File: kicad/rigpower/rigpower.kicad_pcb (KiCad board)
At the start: 2 copper layers, 66 x 54.6 mm, 16 parts, among them J1 Conn_01x02, J2 Conn_01x02, J3 Conn_01x02, J4 Conn_01x02, J5 Conn_01x02

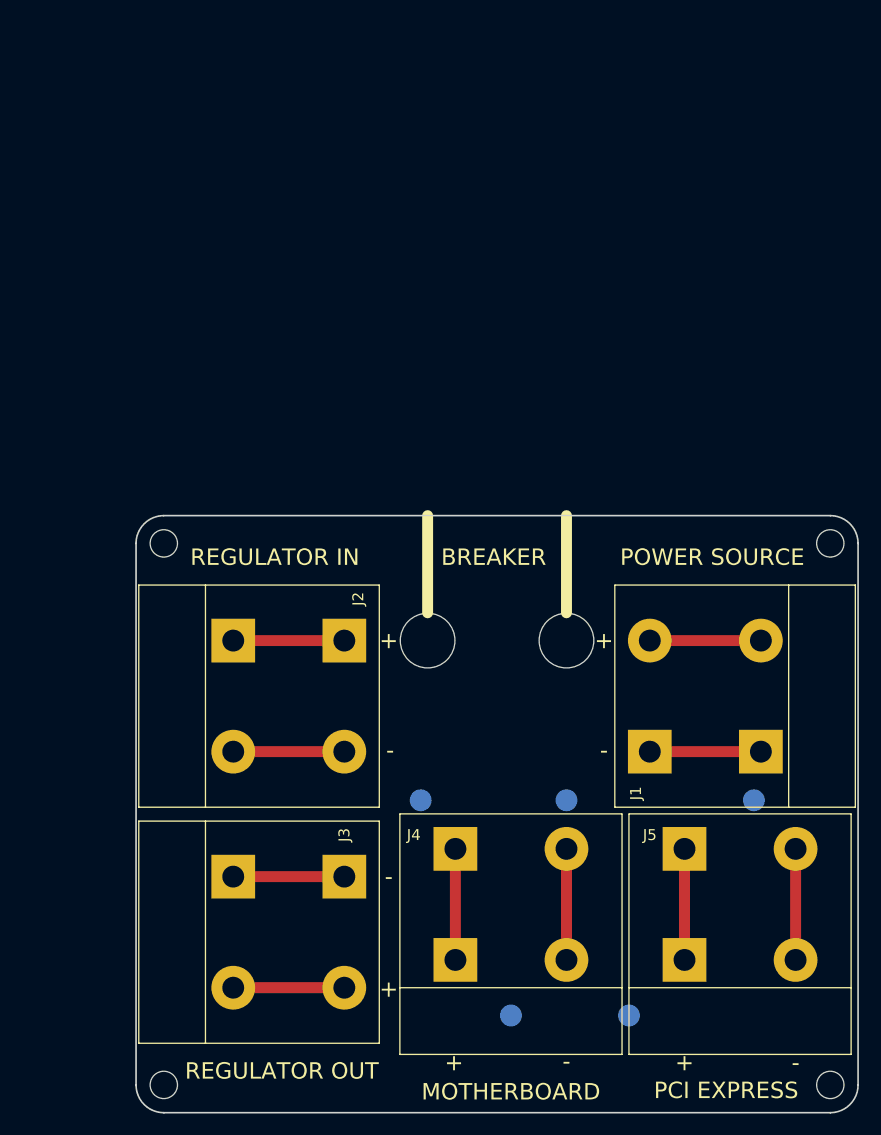
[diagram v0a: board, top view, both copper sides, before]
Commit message: rigpower renewal
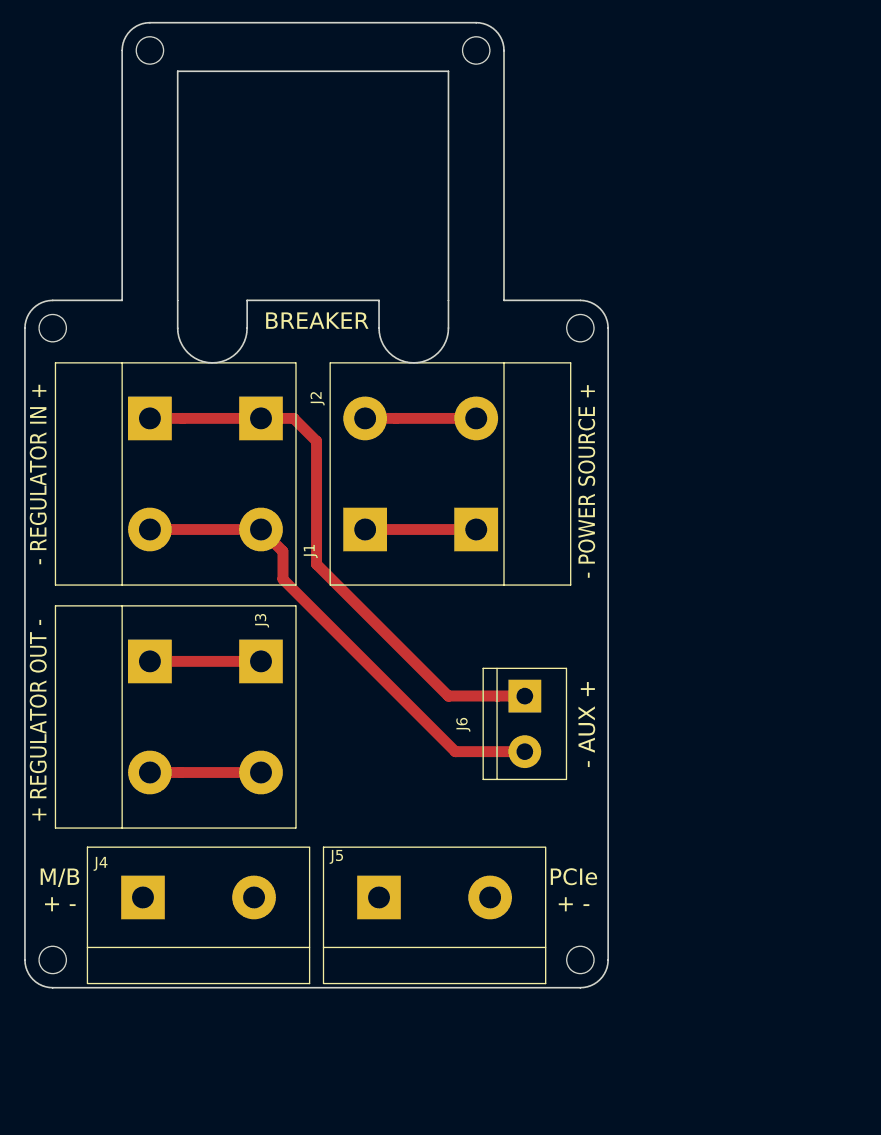
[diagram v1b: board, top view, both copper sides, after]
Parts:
- removed the REF** at (157.5, 111.1)
- removed the REF** at (157.5, 96.5)
- removed the REF** at (163.2, 130.8)
- removed the REF** at (152.4, 130.8)
- removed the REF** at (144.1, 111.1)
- removed the REF** at (174.6, 111.1)
- removed the REF** at (144.8, 96.5)
- added J6: Conn_01x02, TerminalBlock:TerminalBlock_bornier-2_P5.08mm, F.Cu at (153.7, 101.6)
- added REF**: MountingHole_2.5mm, MountingHole:MountingHole_2.5mm, F.Cu at (119.4, 42.5)
- added REF**: MountingHole_2.5mm, MountingHole:MountingHole_2.5mm, F.Cu at (149.2, 42.5)
- J4, J5: footprint lib:TerminalBlock_P10.16mm -> lib:TerminalBlock_P9.5mm
- moved J1 33.0 mm to (149.2, 86.4)
- moved REF** 30.2 mm to (158.8, 67.9)
- moved J4 29.1 mm to (118.7, 120.0)
- moved J5 28.5 mm to (140.3, 120.0)
- moved REF** 25.6 mm to (158.8, 125.7)
- moved REF** 22.2 mm to (110.5, 67.9)
- moved J2 21.7 mm to (119.4, 76.2)
- moved J3 21.1 mm to (119.4, 98.4)
- moved REF** 15.3 mm to (110.5, 125.7)
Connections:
- J4 pad 1: Net-(J4-Pad1) -> (no net)
- J4 pad 2: Net-(J4-Pad2) -> (no net)
- J5 pad 1: Net-(J5-Pad1) -> (no net)
- J5 pad 2: Net-(J5-Pad2) -> (no net)
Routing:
- net Net-(J2-Pad1): track 10.2 -> 51.4 mm
- net Net-(J2-Pad2): track 10.2 -> 44.2 mm
- net Net-(J5-Pad2): track 10.2 -> 0.00 mm
- net Net-(J5-Pad1): track 10.2 -> 0.00 mm
- net Net-(J4-Pad2): track 10.2 -> 0.00 mm
- net Net-(J4-Pad1): track 10.2 -> 0.00 mm
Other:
- board size 66 x 54.6 mm -> 53.3 x 88.3 mm
- board text added: "+ REGULATOR OUT -"
- board text added: "- AUX +"
- board text added: "- POWER SOURCE +"
- board text added: "- REGULATOR IN +"
- board text added: "M/B + -"
- board text added: "PCIe + -"
- board text removed: "+"
- board text removed: "-"
- board text removed: "MOTHERBOARD"
- board text removed: "PCI EXPRESS"
- board text removed: "POWER SOURCE"
- board text removed: "REGULATOR IN"
- board text removed: "REGULATOR OUT"
